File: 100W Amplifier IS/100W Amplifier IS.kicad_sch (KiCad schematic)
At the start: 17 parts, among them U1 TDA7294

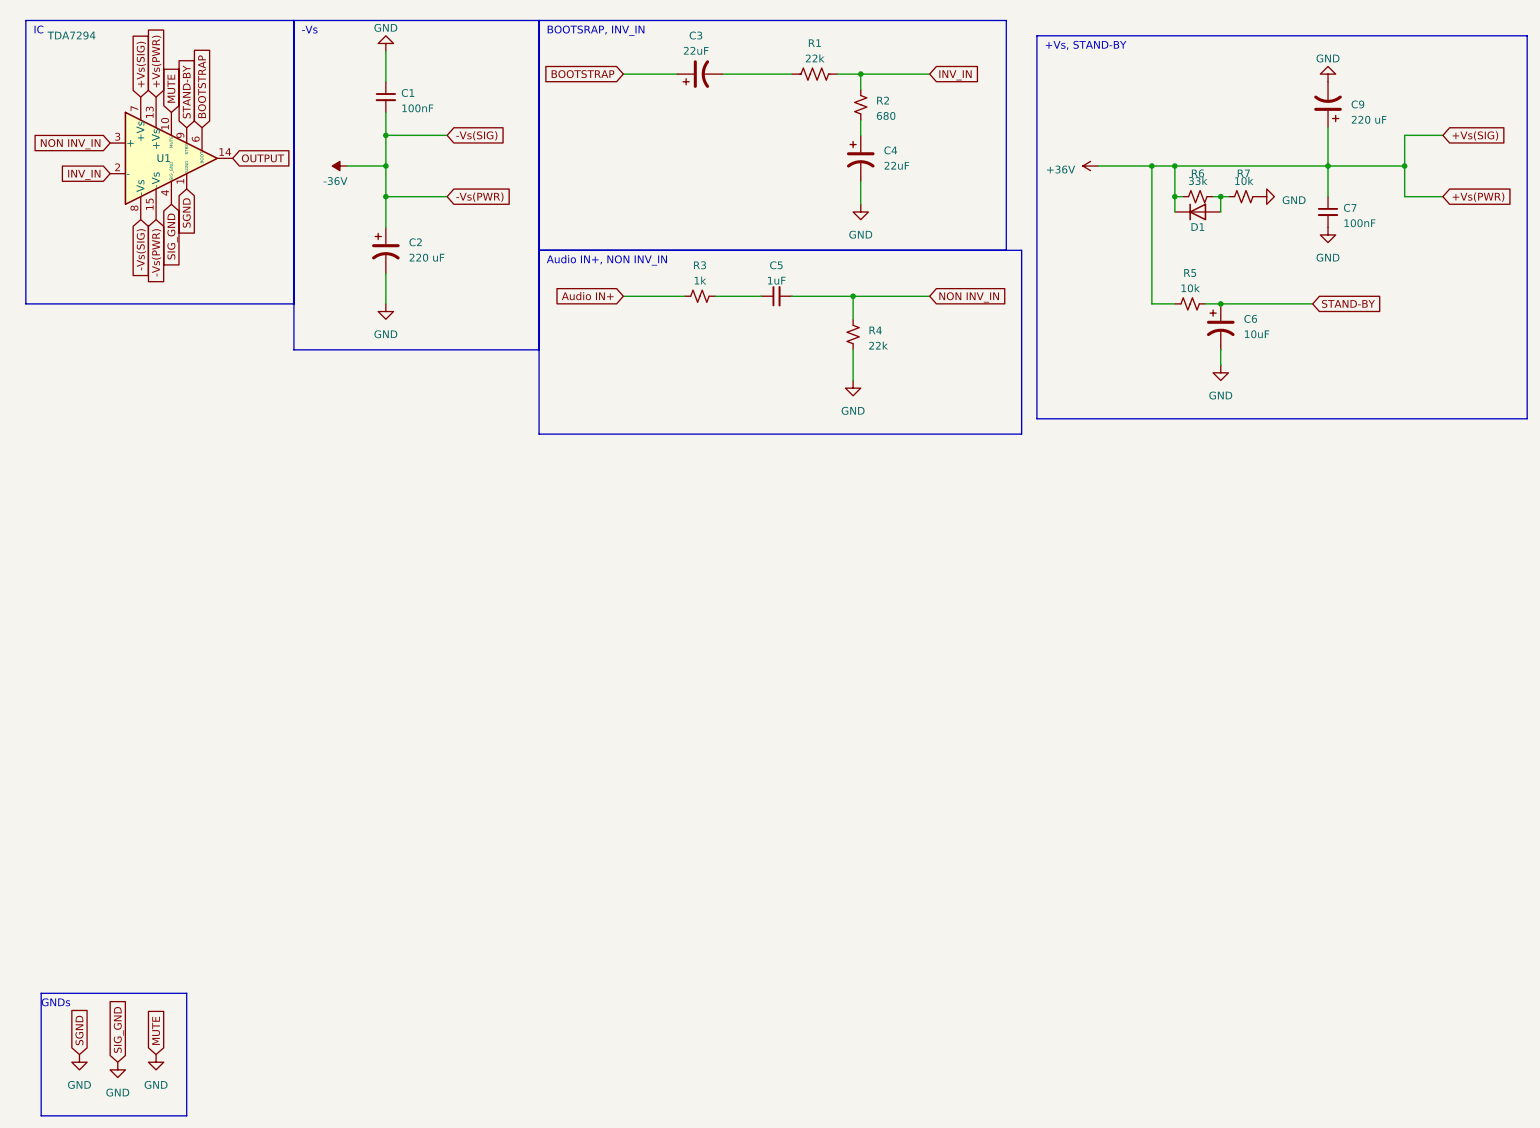
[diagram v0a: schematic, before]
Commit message: New Circuit and KiCad PCB Completed
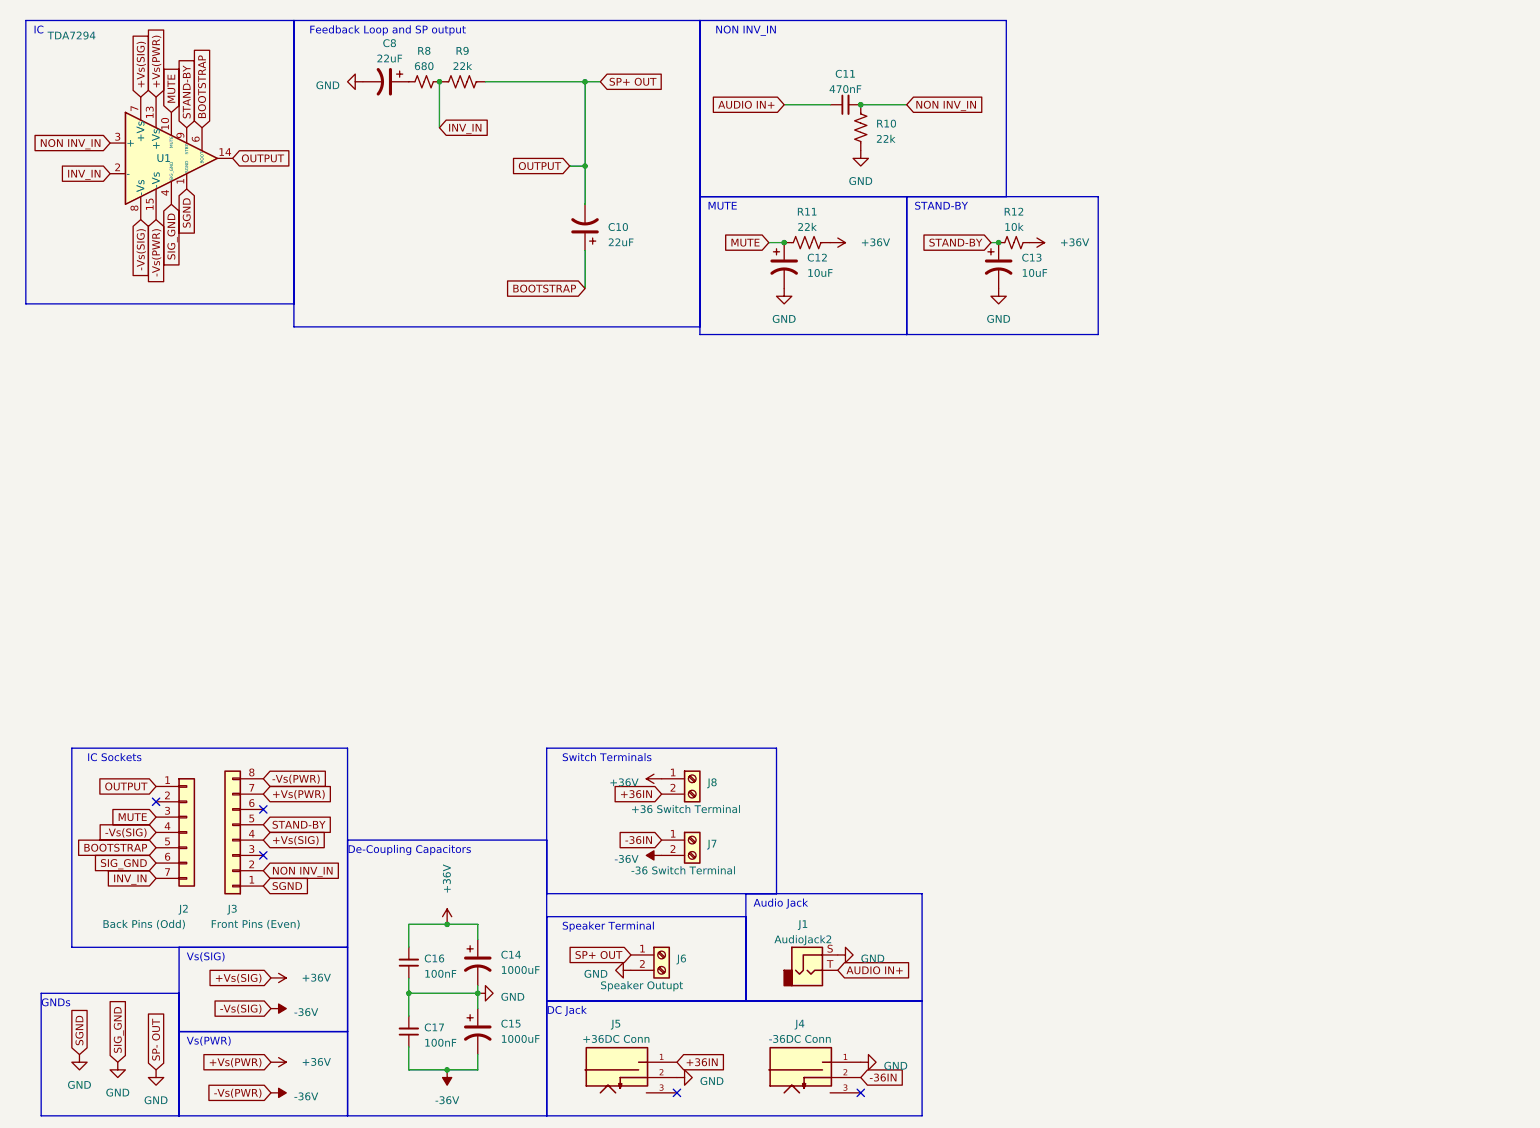
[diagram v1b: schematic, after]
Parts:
- removed C1, C7: 100nF, symbol Device:C_Small
- removed C2, C9: 220 uF, Capacitor_THT:CP_Radial_D12.5mm_P5.00mm, symbol Device:C_Polarized_US
- removed C3, C4: 22uF, Capacitor_THT:CP_Radial_D10.0mm_P5.00mm, symbol Device:C_Polarized_US
- removed C5: 1uF, symbol Device:C_Small
- removed C6: 10uF, Capacitor_THT:CP_Radial_D8.0mm_P3.50mm, symbol Device:C_Polarized_US
- removed D1: ~, Diode_THT:D_DO-35_SOD27_P7.62mm_Horizontal, symbol Diode:1N4148
- removed R1: 22k, symbol Device:R_US
- removed R2: 680, symbol Device:R_Small_US
- removed R3: 1k, symbol Device:R_Small_US
- removed R4: 22k, symbol Device:R_Small_US
- removed R5, R7: 10k, symbol Device:R_Small_US
- removed R6: 33k, symbol Device:R_Small_US
- added C10, C8: 22uF, Capacitor_THT:CP_Radial_D10.0mm_P5.00mm, symbol Device:C_Polarized_US
- added C11: 470nF, Capacitor_THT:C_Disc_D5.0mm_W2.5mm_P5.00mm, symbol Device:C_Small
- added C12, C13: 10uF, Capacitor_THT:CP_Radial_D8.0mm_P3.50mm, symbol Device:C_Polarized_US
- added C14, C15: 1000uF, Capacitor_THT:CP_Radial_D16.0mm_P7.50mm, symbol Device:C_Polarized_US
- added C16, C17: 100nF, Capacitor_THT:C_Disc_D5.0mm_W2.5mm_P5.00mm, symbol Device:C_Small
- added J1: AudioJack2, Connector_Audio:Jack_3.5mm_CUI_SJ1-3523N_Horizontal, symbol Connector_Audio:AudioJack2
- added J2: Back Pins (Odd), Connector_PinSocket_2.54mm:PinSocket_1x07_P2.54mm_Vertical, symbol Connector_Generic:Conn_01x07
- added J3: Front Pins (Even), Connector_PinSocket_2.54mm:PinSocket_1x08_P2.54mm_Vertical, symbol Connector_Generic:Conn_01x08
- added J4: -36DC Conn, CON_SOCJ_2155:GRAVITECH_CON-SOCJ-2155, symbol CON-SOCJ-2155:CON-SOCJ-2155
- added J5: +36DC Conn, CON_SOCJ_2155:GRAVITECH_CON-SOCJ-2155, symbol CON-SOCJ-2155:CON-SOCJ-2155
- added J6: Speaker Outupt, TerminalBlock:TerminalBlock_Altech_AK300-2_P5.00mm, symbol Connector:Screw_Terminal_01x02
- added J7: -36 Switch Terminal, TerminalBlock:TerminalBlock_Altech_AK300-2_P5.00mm, symbol Connector:Screw_Terminal_01x02
- added J8: +36 Switch Terminal, TerminalBlock:TerminalBlock_Altech_AK300-2_P5.00mm, symbol Connector:Screw_Terminal_01x02
- added R10, R11, R9: 22k, Resistor_THT:R_Axial_DIN0207_L6.3mm_D2.5mm_P10.16mm_Horizontal, symbol Device:R_US
- added R12: 10k, Resistor_THT:R_Axial_DIN0207_L6.3mm_D2.5mm_P10.16mm_Horizontal, symbol Device:R_Small_US
- added R8: 680, Resistor_THT:R_Axial_DIN0207_L6.3mm_D2.5mm_P10.16mm_Horizontal, symbol Device:R_Small_US
- U1: footprint Package_TO_SOT_THT:TO-220-15_P2.54x2.54mm_StaggerOdd_Lead4.58mm_Vertical -> (none)
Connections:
- net +36V: now also C14.1, C16.2, J3.4 (Pin_4), J3.7 (Pin_7), J8.1 (Pin_1), R11.1, R12.1
- net -36V: now also C15.2, C17.1, J2.4 (Pin_4), J3.8 (Pin_8), J7.2 (Pin_2)
- net BOOTSTRAP: now also C10.1, J2.5 (Pin_5)
- net GND: now also C12.2, C13.2, C14.2, C15.1, C16.1, C17.2, C8.2, J1.S, J2.6 (Pin_6), J3.1 (Pin_1), J4.1, J5.2, J6.2 (Pin_2), R10.1; no longer U1.10 (MUTE)
- net INV_IN: now also J2.7 (Pin_7), R8.2, R9.1
- net NON INV_IN: now also C11.2, J3.2 (Pin_2), R10.2
- net OUTPUT: now also C10.2, J2.1 (Pin_1), J6.1 (Pin_1), R9.2
- net STAND-BY: now also C13.1, J3.5 (Pin_5), R12.2
- new net: C8.1, R8.1
- new net +36IN: J5.1, J8.2 (Pin_2)
- new net -36IN: J4.2, J7.1 (Pin_1)
- new net AUDIO IN+: C11.1, J1.T
- new net MUTE: C12.1, J2.3 (Pin_3), R11.2, U1.10 (MUTE)
- no-connect marks 0 -> 5
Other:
- note added: "Audio Jack"
- note added: "DC Jack"
- note added: "De-Coupling Capacitors"
- note added: "Feedback Loop and SP output"
- note added: "IC Sockets"
- note added: "MUTE"
- note added: "NON INV_IN"
- note added: "STAND-BY"
- note added: "Speaker Terminal"
- note added: "Switch Terminals"
- note added: "Vs(PWR)"
- note added: "Vs(SIG)"
- note removed: "+Vs, STAND-BY"
- note removed: "-Vs"
- note removed: "Audio IN+, NON INV_IN"
- note removed: "BOOTSRAP, INV_IN"
